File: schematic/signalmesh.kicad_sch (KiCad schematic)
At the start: 52 parts, among them J1 FPGA I/O, J10 INA219_CONFIG, J11 INA219_CONFIG, J12 AAM_DBG, J13 DSM_DBG, J2 FPGA I/O, J4 TDM_DBG, J5 INA219_CONFIG, J6 INA219_CONFIG, J7 INA219_CONFIG, J8 FPGA I/O, J9 FPGA I/O, U1 NUCLEO-H753ZI, U10 INA219AxD, U11 INA219AxD, U12 INA219AxD, U13 INA219AxD, U2 NUCLEO-H753ZI, U3 NUCLEO-F303RE, U4 YAAJ_BluePill_Part_Like, U5 24LC256-I_SN, U6 BME280, U7 INA219AxD, U8 24LC256-I_SN, U9 NUCLEO-F446RE

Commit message: more schematic updates. semiworking PCB
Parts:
- added C6: 10uf, Capacitor_SMD:C_0201_0603Metric, symbol Device:C_Small
- added D10, D11, D5, D6, D7, D8, D9: LED_PWR, LED_SMD:LED_Kingbright_KPBD-3224, symbol Device:LED
- added D12: LED_OK, LED_SMD:LED_Kingbright_KPBD-3224, symbol Device:LED
- added D13: LED_FAIL, LED_SMD:LED_Kingbright_KPBD-3224, symbol Device:LED
- added D14: LED_WARN, LED_SMD:LED_Kingbright_KPBD-3224, symbol Device:LED
- added J14: ACM_DBG, Connector_PinHeader_1.00mm:PinHeader_1x03_P1.00mm_Horizontal, symbol Connector_Generic:Conn_01x03
- added R27, R29, R30, R31, R32, R33, R34, R35, R36, R37: 300, Resistor_SMD:R_0805_2012Metric_Pad1.20x1.40mm_HandSolder, symbol Device:R
- added U14: W25Q128JVS, Package_SO:SOIC-8_5.3x5.3mm_P1.27mm, symbol Memory_Flash:W25Q128JVS
- added U15: AP2112K-3.3, Package_TO_SOT_SMD:SOT-23-5, symbol Regulator_Linear:AP2112K-3.3
- added U16: 74HC4050D, 74HC4050D:SO16, symbol 74HC4050D:74HC4050D
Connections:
- net 3V3_ACM: now also U14.3 (~{WP}/IO_{2}), U14.7 (~{HOLD}/~{RESET}/IO_{3}), U16.1 (VCC)
- net 5V_ACM: now also U10.8 (IN+)
- net 5V_TDM: no longer U10.8 (IN+), U11.8 (IN+), U12.8 (IN+), U13.8 (IN+)
- net GND: now also U3.CN10_20 (GND_S2), U3.CN10_9 (GND_S2), C6.2, D10.1 (K), D11.1 (K), D12.1 (K), D13.1 (K), D14.1 (K), D5.1 (K), D6.1 (K), D7.1 (K), D8.1 (K), D9.1 (K), J14.3 (Pin_3), U14.4 (GND), U15.2 (GND), U16.11 (5A), U16.14 (6A), U16.8 (GND)
- net 5V_UUM: now reaches U3.CN10_8 (U5V)
- net 5V_UUM: now also U12.8 (IN+)
- net I2C1_SCL_TDM renamed TDM_I2C1_SCL
- net I2C1_SDA_TDM renamed TDM_I2C1_SDA
- net IOB11A_PMOD2.2 renamed ACM_LED_PWR
- net IOB11B_PMOD2.1 renamed ACM_LED_WARN
- net ACM_LED_WARN: now also R36.2
- net IOB13A_PMOD2.8 renamed ACM_LED_FAIL
- net ACM_LED_FAIL: now also R37.2
- net IOB13B_PMOD2.7 renamed ACM_LED_OK
- net ACM_LED_OK: now also R35.2
- net IOB29B_PMOD1.2 renamed ACM_SPI_SCLK
- net ACM_SPI_SCLK: now also U16.5 (2A)
- net IOB31A_PMOD1.3 renamed ACM_SPI_MOSI
- net ACM_SPI_MOSI: now also U16.7 (3A)
- net IOB31B_PMOD1.4 renamed ACM_SPI_CS
- net ACM_SPI_CS: now also U16.3 (1A)
- net IOB33A_PMOD1.1 renamed ACM_SPI_MISO
- net ACM_SPI_MISO: now also U16.9 (4A)
- net IOB8A_PMOD2.4 renamed ACM_DBG_TX
- net ACM_DBG_TX: now also J14.1 (Pin_1)
- net IOB8B_PMOD2.3 renamed ACM_DBG_RX
- net ACM_DBG_RX: now also J14.2 (Pin_2)
- net LEDFAIL_TDM renamed TDM_LED_FAIL
- net LEDOK_TDM renamed TDM_LED_OK
- net LEDWARN_TDM renamed TDM_LED_WARN
- net VDD_TDM renamed TDM_VDD
- net TDM_VDD: now also R27.2; no longer U10.7 (IN-), U11.7 (IN-), U12.7 (IN-), U13.7 (IN-)
- new net: D7.2 (A), R30.1
- new net: D12.2 (A), R35.1
- new net: D10.2 (A), R33.2
- new net: D13.2 (A), R36.1
- new net: U14.1 (~{CS}), U16.2 (1Y)
- new net: U14.2 (DO/IO_{1}), U16.10 (4Y)
- new net: U14.5 (DI/IO_{0}), U16.6 (3Y)
- new net: U14.6 (CLK), U16.4 (2Y)
- new net: C6.1, R33.1, U14.8 (VCC), U15.5 (VOUT)
- new net: D8.2 (A), R31.1
- new net: D6.2 (A), R29.1
- new net: D11.2 (A), R34.1
- new net: D14.2 (A), R37.1
- new net: D9.2 (A), R32.1
- new net: D5.2 (A), R27.1
- new net 5V_AAM: U13.8 (IN+)
- new net 5V_DSM: U11.8 (IN+)
- new net ACM_VDD: R34.2
- new net VDD_AAM: R30.2, U13.7 (IN-)
- new net VDD_ACM: R29.2, U10.7 (IN-), U15.1 (VIN), U15.3 (EN)
- new net VDD_DSM: R32.2, U11.7 (IN-)
- new net VDD_UUM: R31.2, U12.7 (IN-)
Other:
- note added: "Audio Creation Module"
- note added: "Upload & Update Module"
- note added: "W25Q128 ACM"
- moved on the sheet: C1, C2, C3, C4, C5, D1, D2, D3, D4, J1, J10, J11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

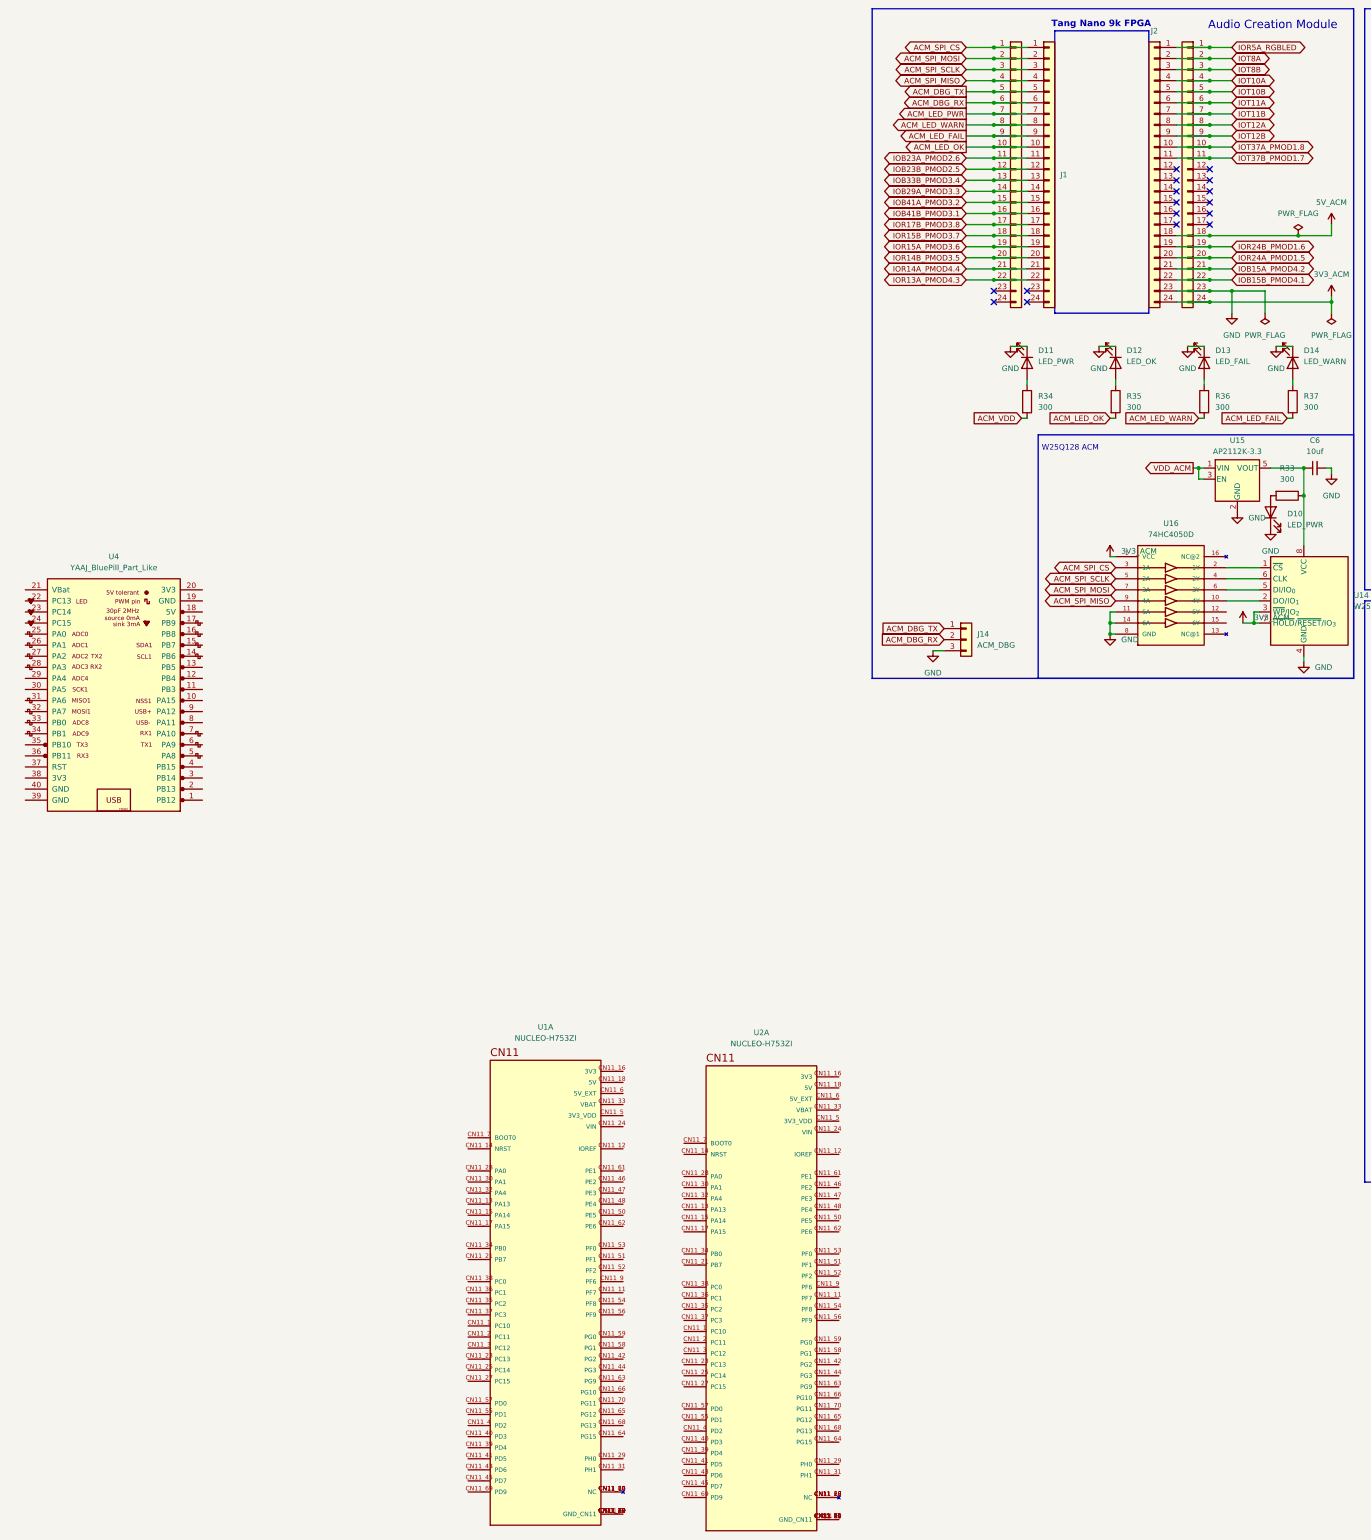
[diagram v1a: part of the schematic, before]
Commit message: more schematic updates. semiworking PCB
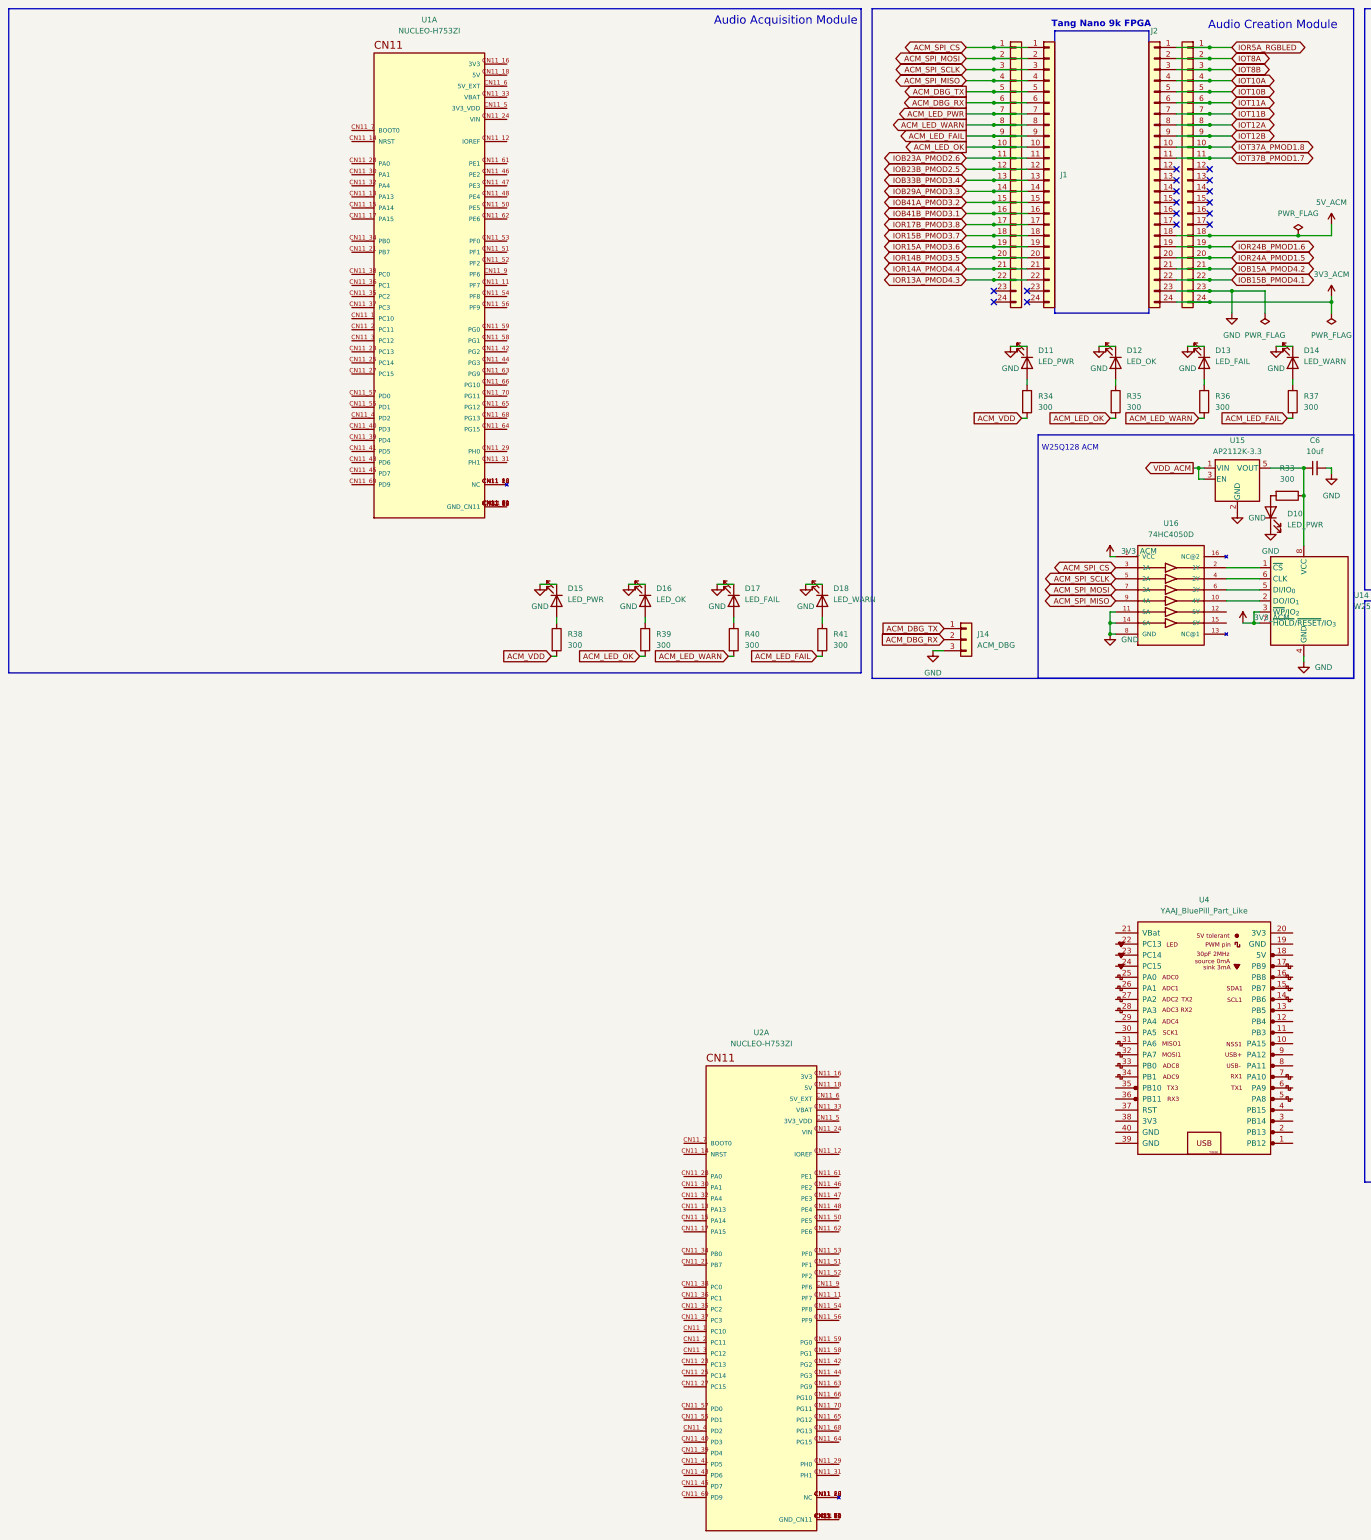
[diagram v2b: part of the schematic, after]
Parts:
- added D15: LED_PWR, LED_SMD:LED_Kingbright_KPBD-3224, symbol Device:LED
- added D16: LED_OK, LED_SMD:LED_Kingbright_KPBD-3224, symbol Device:LED
- added D17: LED_FAIL, LED_SMD:LED_Kingbright_KPBD-3224, symbol Device:LED
- added D18: LED_WARN, LED_SMD:LED_Kingbright_KPBD-3224, symbol Device:LED
- added R38, R39, R40, R41: 300, Resistor_SMD:R_0805_2012Metric_Pad1.20x1.40mm_HandSolder, symbol Device:R
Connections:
- net ACM_LED_FAIL: now also R41.2
- net ACM_LED_OK: now also R39.2
- net ACM_LED_WARN: now also R40.2
- net ACM_VDD: now also R38.2
- net GND: now also D15.1 (K), D16.1 (K), D17.1 (K), D18.1 (K)
- new net: D17.2 (A), R40.1
- new net: D15.2 (A), R38.1
- new net: D18.2 (A), R41.1
- new net: D16.2 (A), R39.1
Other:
- note added: "Audio Acquisition Module"
- moved on the sheet: U1A, U4
